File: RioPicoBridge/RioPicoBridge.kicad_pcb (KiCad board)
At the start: 2 copper layers, 56.7 x 77.5 mm, 19 parts, among them J1 DUPONT, J2 DUPONT, J3 JST, J4 JST, J5 MXP, U1 Pico, U2 LM1117-3.3

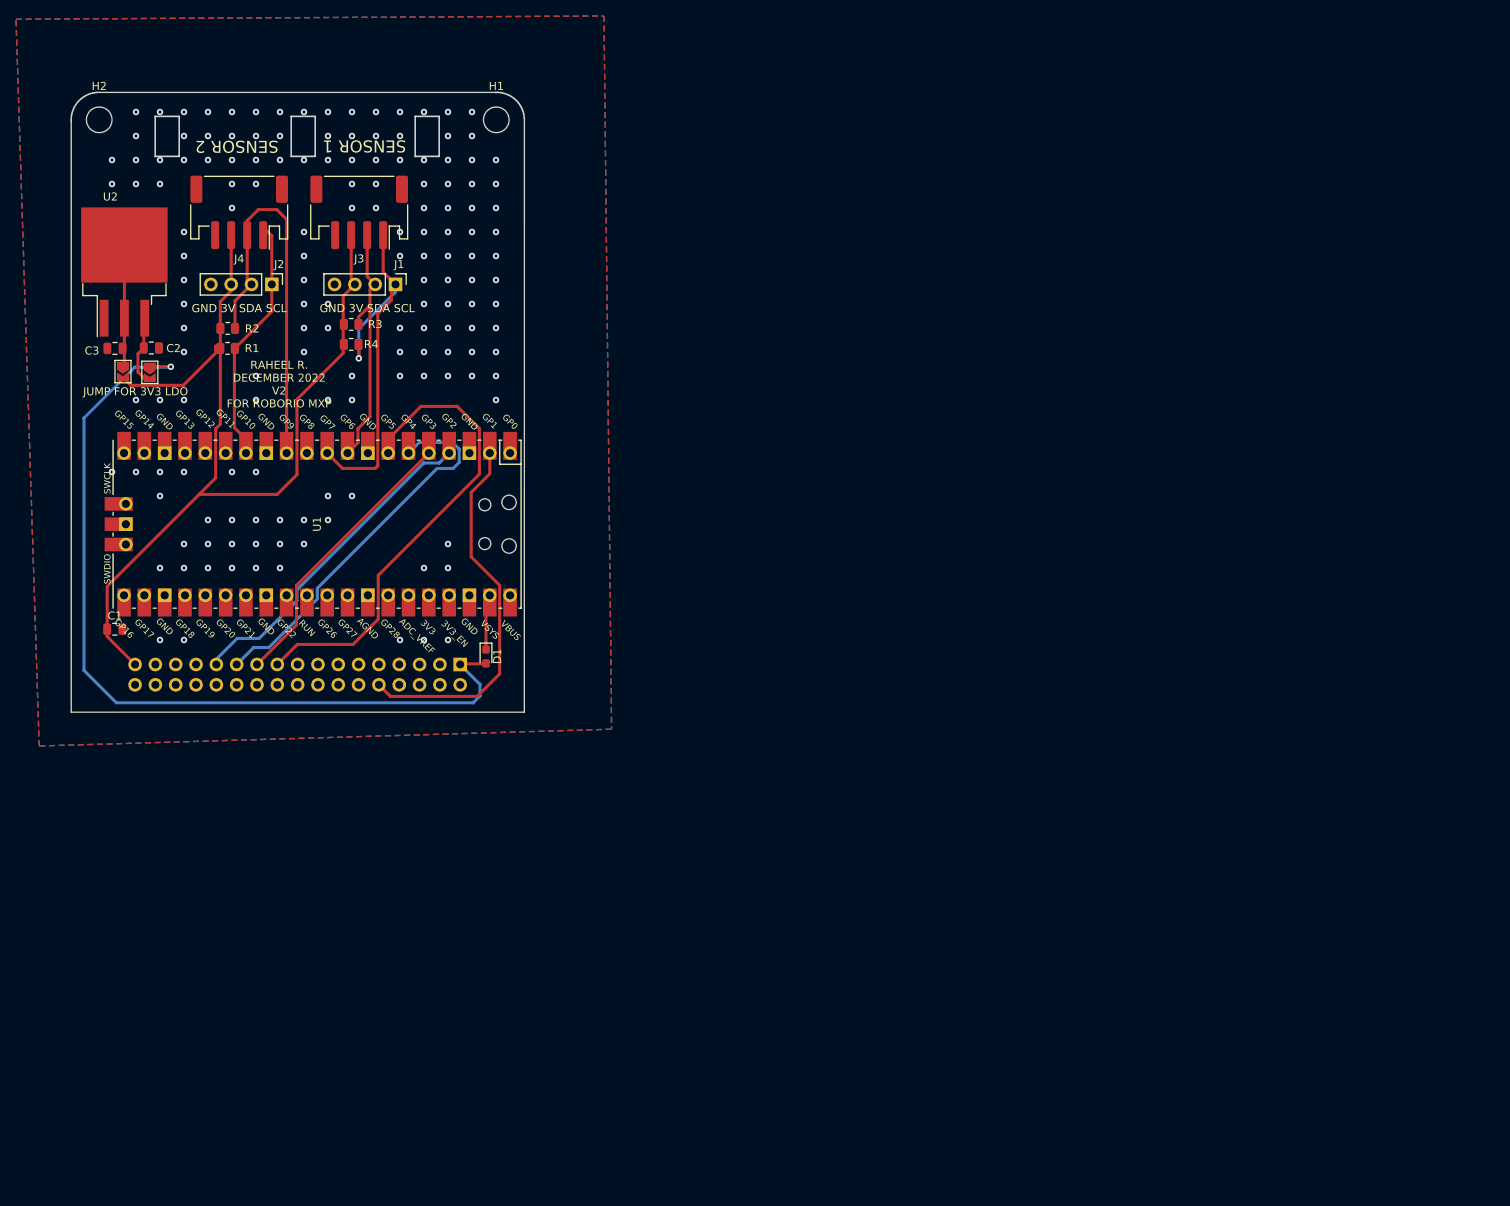
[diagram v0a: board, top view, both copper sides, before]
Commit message: forgot to add gerbers
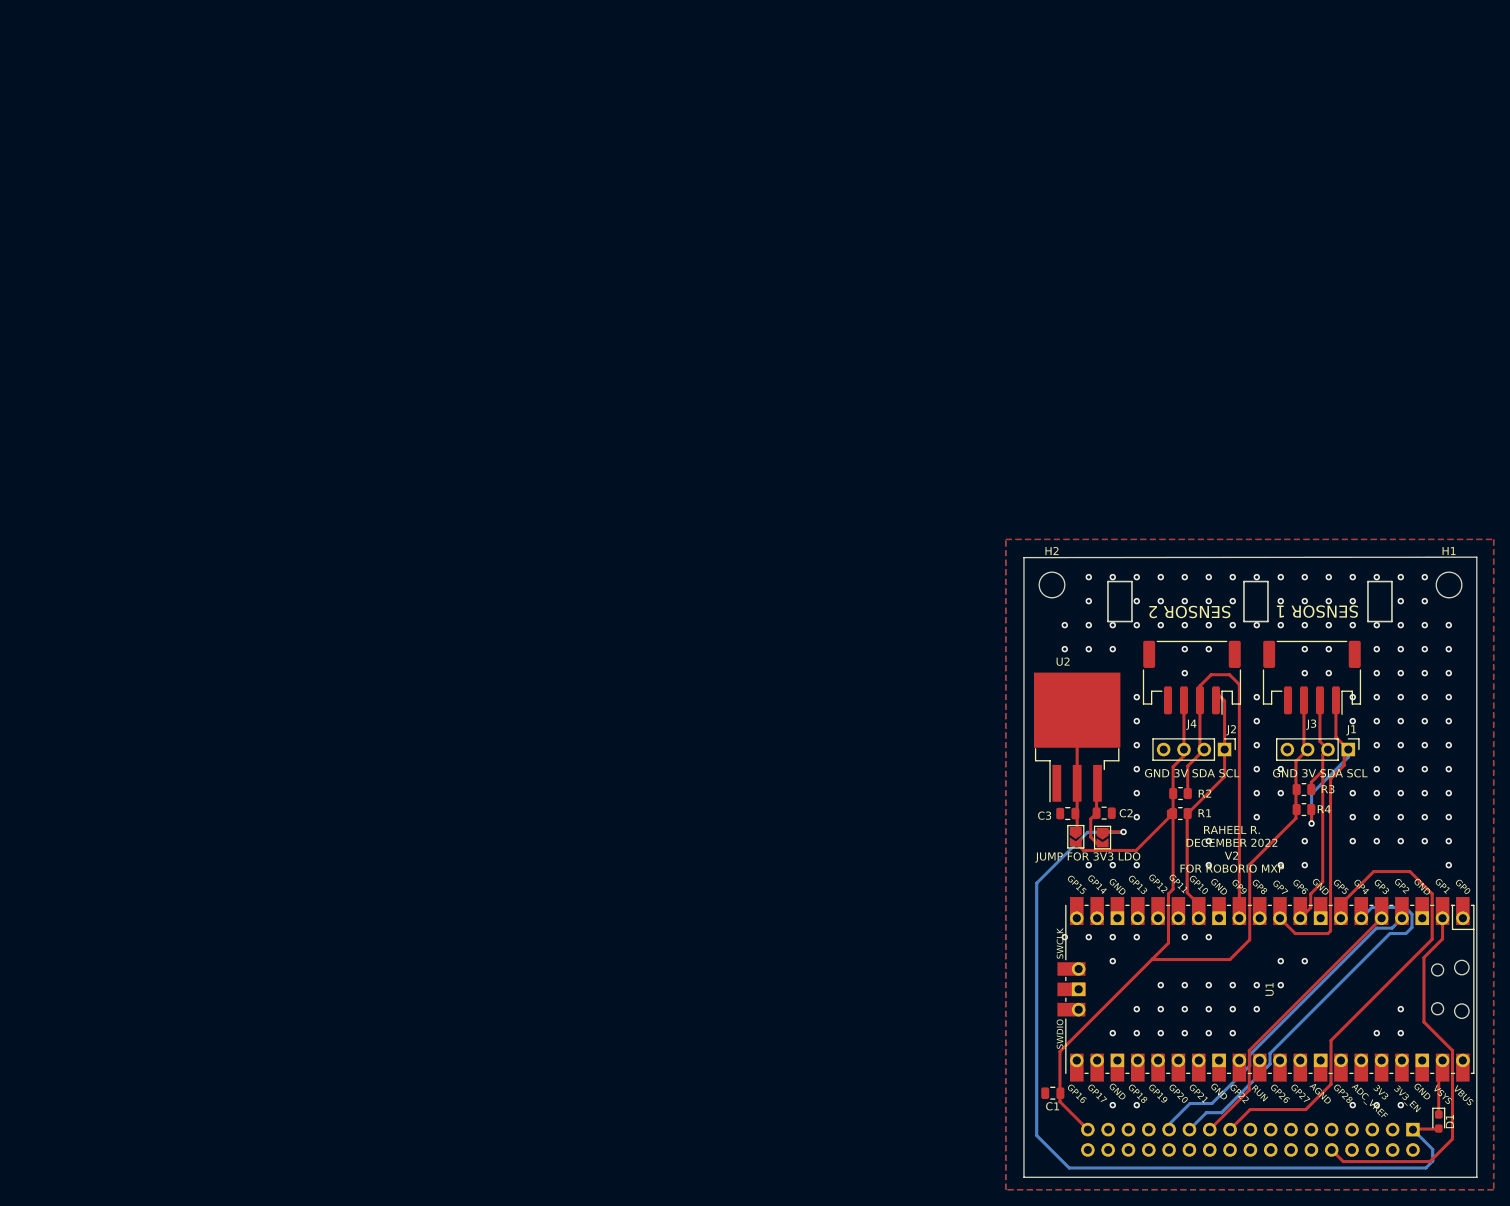
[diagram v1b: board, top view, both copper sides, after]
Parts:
- moved C3 132.5 mm to (124.6, 90.1)
- moved J2 132.5 mm to (144.2, 82.1)
- moved JP1 132.5 mm to (128.9, 93.1)
- moved R1 132.5 mm to (138.6, 90.1)
- moved C2 132.5 mm to (129.1, 90.1)
- moved H1 132.5 mm to (172.2, 61.6)
- moved H2 132.5 mm to (122.6, 61.6)
- moved J1 132.5 mm to (159.6, 82.1)
- moved J3 132.5 mm to (155.1, 73.1)
- moved J4 132.5 mm to (140.1, 73.1)
- moved J5 132.5 mm to (167.7, 129.7)
- moved JP2 132.5 mm to (125.6, 93.0)
- moved R2 132.5 mm to (138.7, 87.6)
- moved R3 132.5 mm to (154.1, 87.1)
- moved R4 132.5 mm to (154.1, 89.6)
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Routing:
- net /SCL2: track 32.1 -> 31.2 mm
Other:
- board size 56.7 x 77.5 mm -> 56.6 x 77.5 mm
